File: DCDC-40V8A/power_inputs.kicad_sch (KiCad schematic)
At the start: 29 parts, among them Q66 2N7002, Q69 Si7141DP, Q70 Si7141DP, Q71 2N7002, Q72 2N7002, Q73 Si7141DP, Q74 Si7141DP, Q75 2N7002

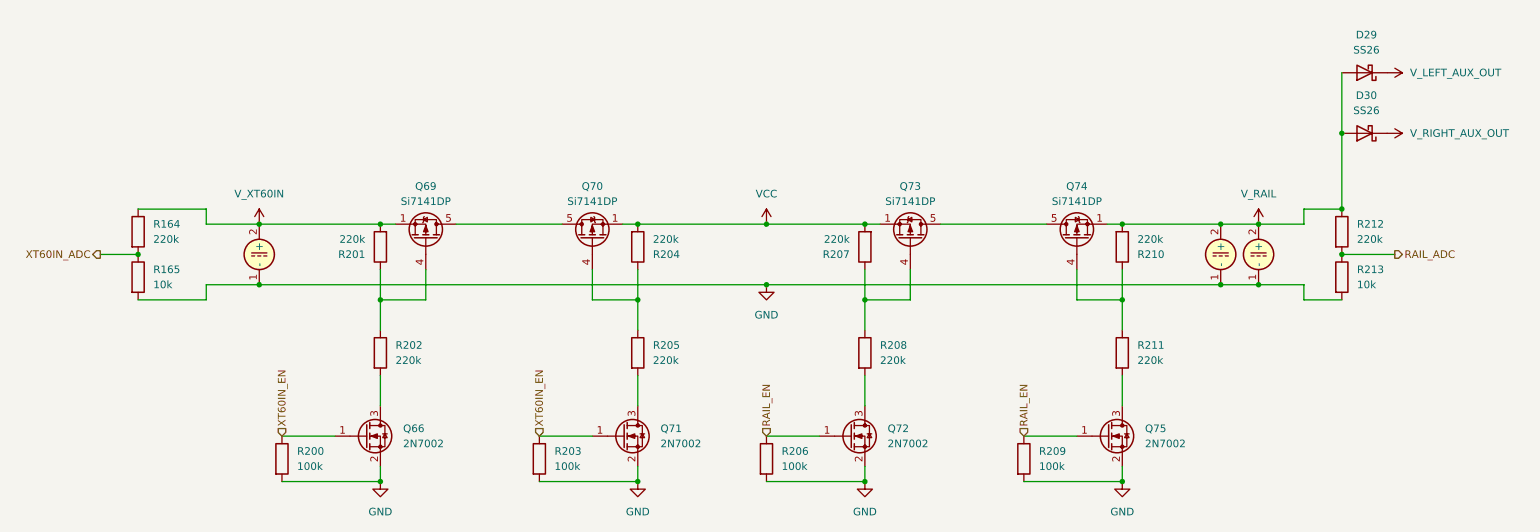
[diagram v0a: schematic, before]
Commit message: wip before CP deletion
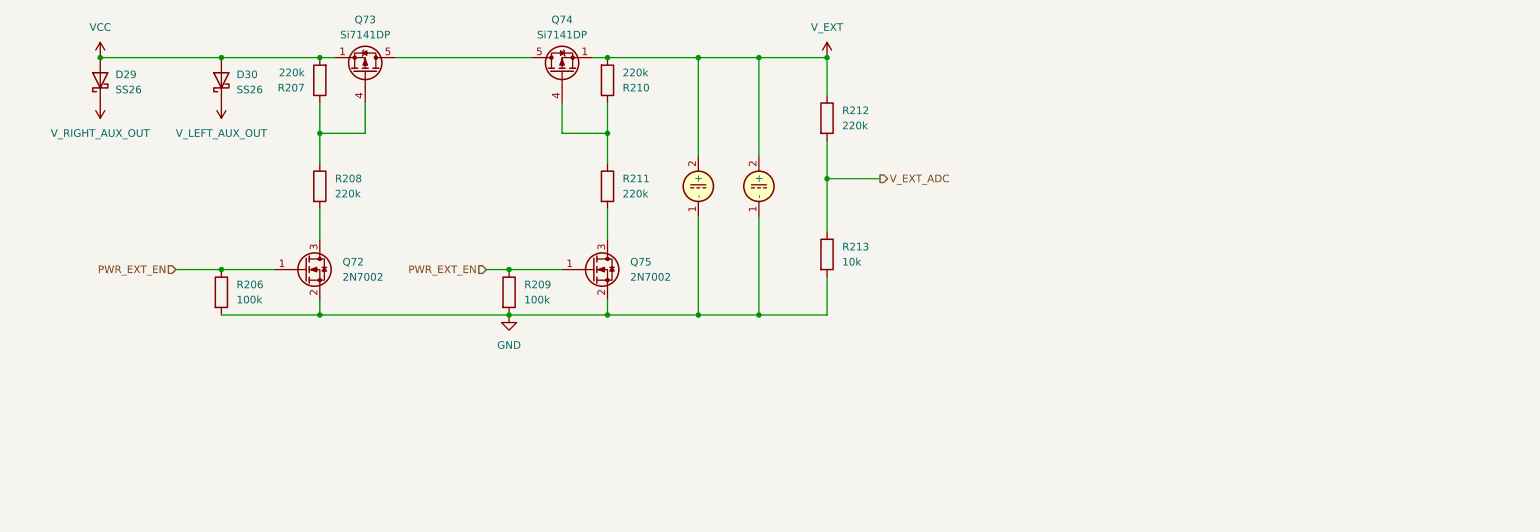
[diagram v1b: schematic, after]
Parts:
- removed Q66, Q71: 2N7002, Package_TO_SOT_SMD:SOT-23, symbol Transistor_FET:2N7002
- removed Q69, Q70: Si7141DP, Package_SO:PowerPAK_SO-8_Single, symbol Transistor_FET:Si7141DP
- removed R164, R201, R202, R204, R205: 220k, Resistor_SMD:R_0402_1005Metric, symbol Device:R
- removed R165: 10k, Resistor_SMD:R_0402_1005Metric, symbol Device:R
- removed R200, R203: 100k, Resistor_SMD:R_0402_1005Metric, symbol Device:R
- removed U14: (no value), Connector_AMASS:AMASS_XT60PW-M_1x02_P7.20mm_Horizontal, symbol DCDC_custom:VDC_XTxx
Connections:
- net VCC: now also D29.2 (A), D30.2 (A)
- net V_LEFT_AUX_OUT: now also D30.1 (K); no longer D29.1 (K)
- net V_RIGHT_AUX_OUT: now also D29.1 (K); no longer D30.1 (K)
- net RAIL_ADC renamed V_EXT_ADC
- net RAIL_EN renamed PWR_EXT_EN
- net V_RAIL renamed V_EXT
- net V_EXT: no longer D29.2 (A), D30.2 (A)
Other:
- moved on the sheet: Q72, Q73, Q74, Q75, R206, R207, R208, R209, R210, R211, R212, R213
